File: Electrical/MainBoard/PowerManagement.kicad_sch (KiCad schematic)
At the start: 73 parts, among them Q1 AO3401A, U5 TPS65131RGE, U6 TPS2121RUXR, U7 TPS7A9401DSCR, U8 LM61460AASQRJRRQ1

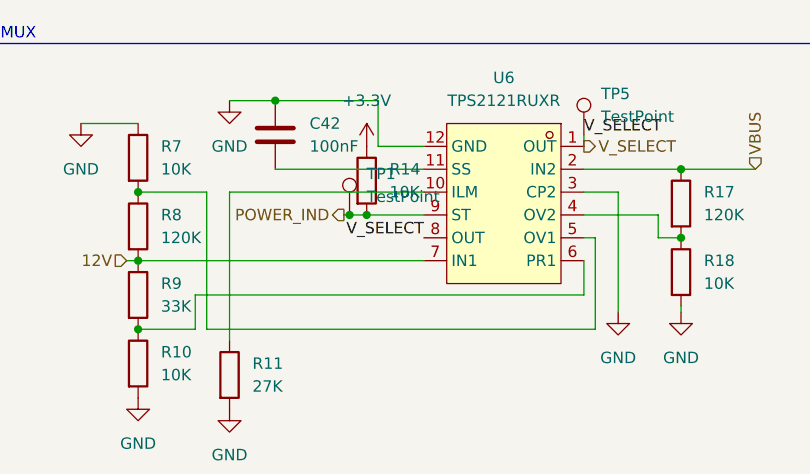
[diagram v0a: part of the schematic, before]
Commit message: manufactured
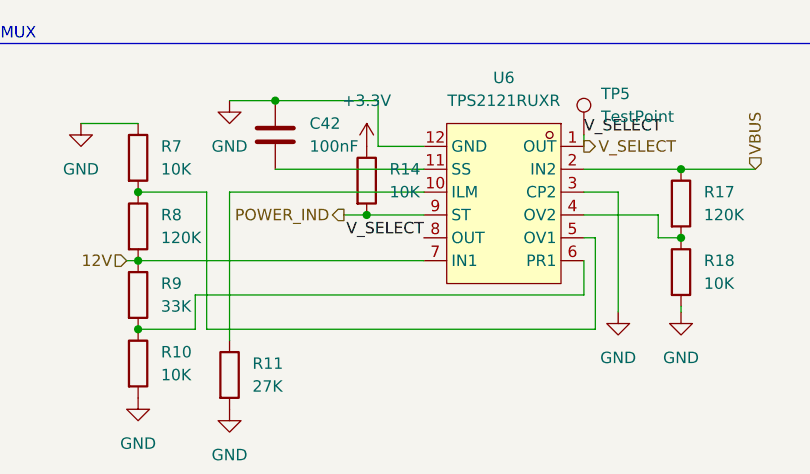
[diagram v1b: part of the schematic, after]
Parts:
- removed TP1: TestPoint, TestPoint:TestPoint_Pad_D2.5mm, symbol Connector:TestPoint
- TP2, TP3, TP4, TP5: footprint TestPoint:TestPoint_Pad_D2.5mm -> TestPoint:TestPoint_Pad_D2.0mm
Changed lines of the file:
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@@
 	)
 	(junction
-		(at 61.595 35.56)
-		(diameter 0)
-		(color 0 0 0 0)
-	)
-	(junction
 		(at 252.095 46.99)
 		(diameter 0)
@@
 	(wire
 		(pts
-			(xy 61.595 35.56) (xy 63.5 35.56)
+			(xy 60.96 35.56) (xy 63.5 35.56)
 		)
 		(stroke
@@
 	(wire
 		(pts
-			(xy 60.96 35.56) (xy 61.595 35.56)
-		)
-		(stroke
-			(width 0)
-			(type default)
-		)
-	)
-	(wire
-		(pts
 			(xy 78.105 95.885) (xy 86.995 95.885)
 		)
@@
 			)
 		)
-		(property "Footprint" "TestPoint:TestPoint_Pad_D2.5mm"
+		(property "Footprint" "TestPoint:TestPoint_Pad_D2.0mm"
 			(at 106.045 76.835 0)
 			(effects
@@
 			)
 		)
-		(property "Footprint" "TestPoint:TestPoint_Pad_D2.5mm"
+		(property "Footprint" "TestPoint:TestPoint_Pad_D2.0mm"
 			(at 92.71 26.67 0)
 			(effects
@@
 			)
 		)
-		(property "Footprint" "TestPoint:TestPoint_Pad_D2.5mm"
+		(property "Footprint" "TestPoint:TestPoint_Pad_D2.0mm"
 			(at 112.395 123.825 0)
 			(effects
@@
 	)
 	(symbol
-		(lib_id "Connector:TestPoint")
-		(at 61.595 35.56 0)
-		(unit 1)
-		(exclude_from_sim no)
-		(in_bom yes)
-		(on_board yes)
-		(dnp no)
-		(fields_autoplaced yes)
-		(property "Reference" "TP1"
-			(at 63.5 30.9879 0)
-			(effects
-				(font
-					(size 1.27 1.27)
-				)
-				(justify left)
-			)
-		)
-		(property "Value" "TestPoint"
-			(at 63.5 33.5279 0)
-			(effects
-				(font
-					(size 1.27 1.27)
-				)
-				(justify left)
-			)
-		)
-		(property "Footprint" "TestPoint:TestPoint_Pad_D2.5mm"
-			(at 66.675 35.56 0)
-			(effects
-				(font
-					(size 1.27 1.27)
-				)
-				(hide yes)
-			)
-		)
-		(property "Datasheet" "~"
-			(at 66.675 35.56 0)
-			(effects
-				(font
-					(size 1.27 1.27)
-				)
-				(hide yes)
-			)
-		)
-		(property "Description" "test point"
-			(at 61.595 35.56 0)
-			(effects
-				(font
-					(size 1.27 1.27)
-				)
-				(hide yes)
-			)
-		)
-		(pin "1"
-		)
-		(instances
-			(project ""
-				(path "/1061c21d-11bf-48d7-8db8-deedefa943c2/7d6e0902-de5f-4868-b5e7-4184774ee025"
-					(reference "TP1")
-					(unit 1)
-				)
-			)
-		)
-	)
-	(symbol
 		(lib_id "Device:R")
 		(at 210.185 60.96 0)
@@
 			)
 		)
-		(property "Footprint" "TestPoint:TestPoint_Pad_D2.5mm"
+		(property "Footprint" "TestPoint:TestPoint_Pad_D2.0mm"
 			(at 259.715 46.99 0)
 			(effects

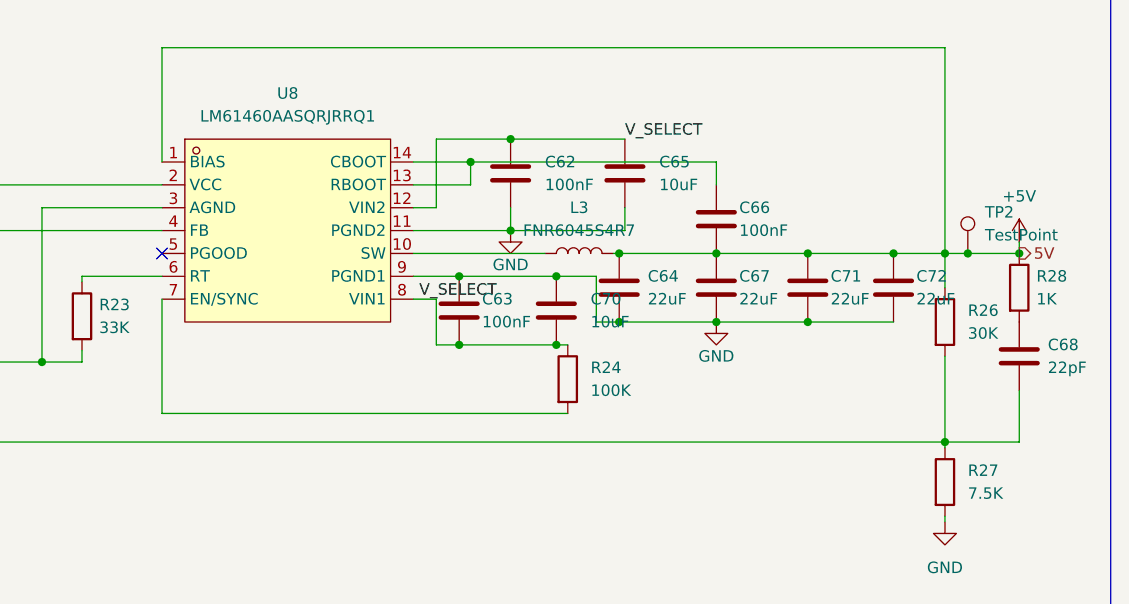
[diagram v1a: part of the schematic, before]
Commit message: software unit testing
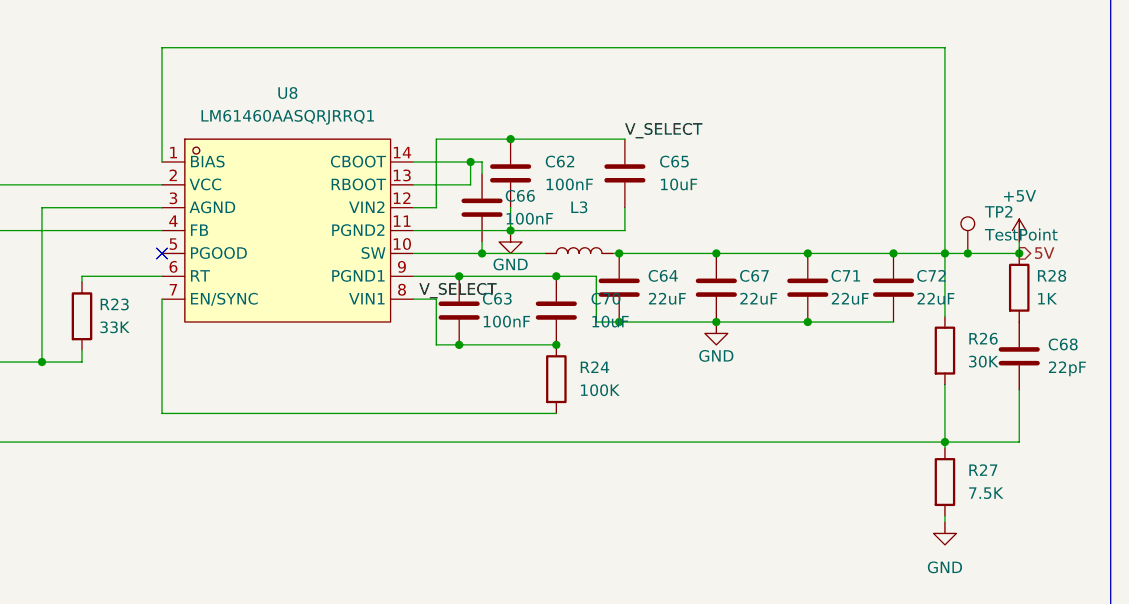
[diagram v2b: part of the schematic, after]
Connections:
- net +5V: no longer C66.2
- net at L3.1, U8.10 (SW): now also C66.2
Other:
- moved on the sheet: C66, R24, R26
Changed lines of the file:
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@@
 	)
 	(junction
+		(at 200.66 46.99)
+		(diameter 0)
+		(color 0 0 0 0)
+	)
+	(junction
 		(at 38.1 40.64)
 		(diameter 0)
@@
 	(wire
 		(pts
-			(xy 208.915 57.15) (xy 210.185 57.15)
-		)
-		(stroke
-			(width 0)
-			(type default)
-		)
-	)
-	(wire
-		(pts
 			(xy 94.615 160.02) (xy 94.615 162.56)
 		)
@@
 	(wire
 		(pts
-			(xy 226.695 36.83) (xy 199.39 36.83)
+			(xy 200.66 36.83) (xy 199.39 36.83)
 		)
 		(stroke
@@
 	(wire
 		(pts
-			(xy 226.695 39.37) (xy 226.695 36.83)
+			(xy 200.66 38.1) (xy 200.66 36.83)
 		)
 		(stroke
@@
 	(wire
 		(pts
+			(xy 200.66 46.99) (xy 207.645 46.99)
+		)
+		(stroke
+			(width 0)
+			(type default)
+		)
+	)
+	(wire
+		(pts
 			(xy 84.455 123.825) (xy 93.98 123.825)
 		)
@@
 	(wire
 		(pts
-			(xy 193.04 46.99) (xy 207.645 46.99)
+			(xy 193.04 46.99) (xy 200.66 46.99)
 		)
 		(stroke
@@
 	(wire
 		(pts
-			(xy 252.095 58.42) (xy 252.095 67.945)
+			(xy 252.095 61.595) (xy 252.095 67.945)
 		)
 		(stroke
@@
 	(wire
 		(pts
-			(xy 165.1 64.77) (xy 210.185 64.77)
+			(xy 165.1 64.77) (xy 208.915 64.77)
 		)
 		(stroke
@@
 	(wire
 		(pts
-			(xy 252.095 50.8) (xy 252.095 46.99)
+			(xy 252.095 53.975) (xy 252.095 46.99)
 		)
 		(stroke
@@
 	(wire
 		(pts
+			(xy 200.66 45.72) (xy 200.66 46.99)
+		)
+		(stroke
+			(width 0)
+			(type default)
+		)
+	)
+	(wire
+		(pts
 			(xy 93.98 111.125) (xy 93.98 116.205)
 		)
@@
 					(size 1.27 1.27)
 				)
+				(hide yes)
 			)
 		)
@@
 	(symbol
 		(lib_id "Device:R")
-		(at 210.185 60.96 0)
+		(at 208.915 60.96 0)
 		(unit 1)
 		(exclude_from_sim no)
@@
 		(fields_autoplaced yes)
 		(property "Reference" "R24"
-			(at 212.725 59.6899 0)
+			(at 211.455 59.6899 0)
 			(effects
 				(font
@@
 		)
 		(property "Value" "100K"
-			(at 212.725 62.2299 0)
+			(at 211.455 62.2299 0)
 			(effects
 				(font
@@
 		)
 		(property "Footprint" "Resistor_SMD:R_0402_1005Metric"
-			(at 208.407 60.96 90)
+			(at 207.137 60.96 90)
 			(effects
 				(font
@@
 		)
 		(property "Datasheet" "~"
-			(at 210.185 60.96 0)
+			(at 208.915 60.96 0)
 			(effects
 				(font
@@
 		)
 		(property "Description" "Resistor"
-			(at 210.185 60.96 0)
+			(at 208.915 60.96 0)
 			(effects
 				(font
@@
 	(symbol
 		(lib_id "Device:R")
-		(at 252.095 54.61 0)
+		(at 252.095 57.785 0)
 		(unit 1)
 		(exclude_from_sim no)
@@
 		(fields_autoplaced yes)
 		(property "Reference" "R26"
-			(at 254.635 53.3399 0)
+			(at 254.635 56.5149 0)
 			(effects
 				(font
@@
 		)
 		(property "Value" "30K"
-			(at 254.635 55.8799 0)
+			(at 254.635 59.0549 0)
 			(effects
 				(font
@@
 		)
 		(property "Footprint" "Resistor_SMD:R_0603_1608Metric"
-			(at 250.317 54.61 90)
+			(at 250.317 57.785 90)
 			(effects
 				(font
@@
 		)
 		(property "Datasheet" "~"
-			(at 252.095 54.61 0)
+			(at 252.095 57.785 0)
 			(effects
 				(font
@@
 		)
 		(property "Description" "Resistor"
-			(at 252.095 54.61 0)
+			(at 252.095 57.785 0)
 			(effects
 				(font
@@
 	(symbol
 		(lib_id "Device:C")
-		(at 226.695 43.18 0)
+		(at 200.66 41.91 0)
 		(unit 1)
 		(exclude_from_sim no)
@@
 		(dnp no)
 		(property "Reference" "C66"
-			(at 229.235 41.91 0)
+			(at 203.2 40.64 0)
 			(effects
 				(font
@@
 		)
 		(property "Value" "100nF"
-			(at 229.235 44.45 0)
+			(at 203.2 43.18 0)
 			(effects
 				(font
@@
 		)
 		(property "Footprint" "Capacitor_SMD:C_0402_1005Metric"
-			(at 227.6602 46.99 0)
+			(at 201.6252 45.72 0)
 			(effects
 				(font
@@
 		)
 		(property "Datasheet" "~"
-			(at 226.695 43.18 0)
+			(at 200.66 41.91 0)
 			(effects
 				(font
@@
 		)
 		(property "Description" "Unpolarized capacitor"
-			(at 226.695 43.18 0)
+			(at 200.66 41.91 0)
 			(effects
 				(font
